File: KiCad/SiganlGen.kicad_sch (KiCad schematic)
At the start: 1 part, among them J1 Barrel_Jack_MountingPin

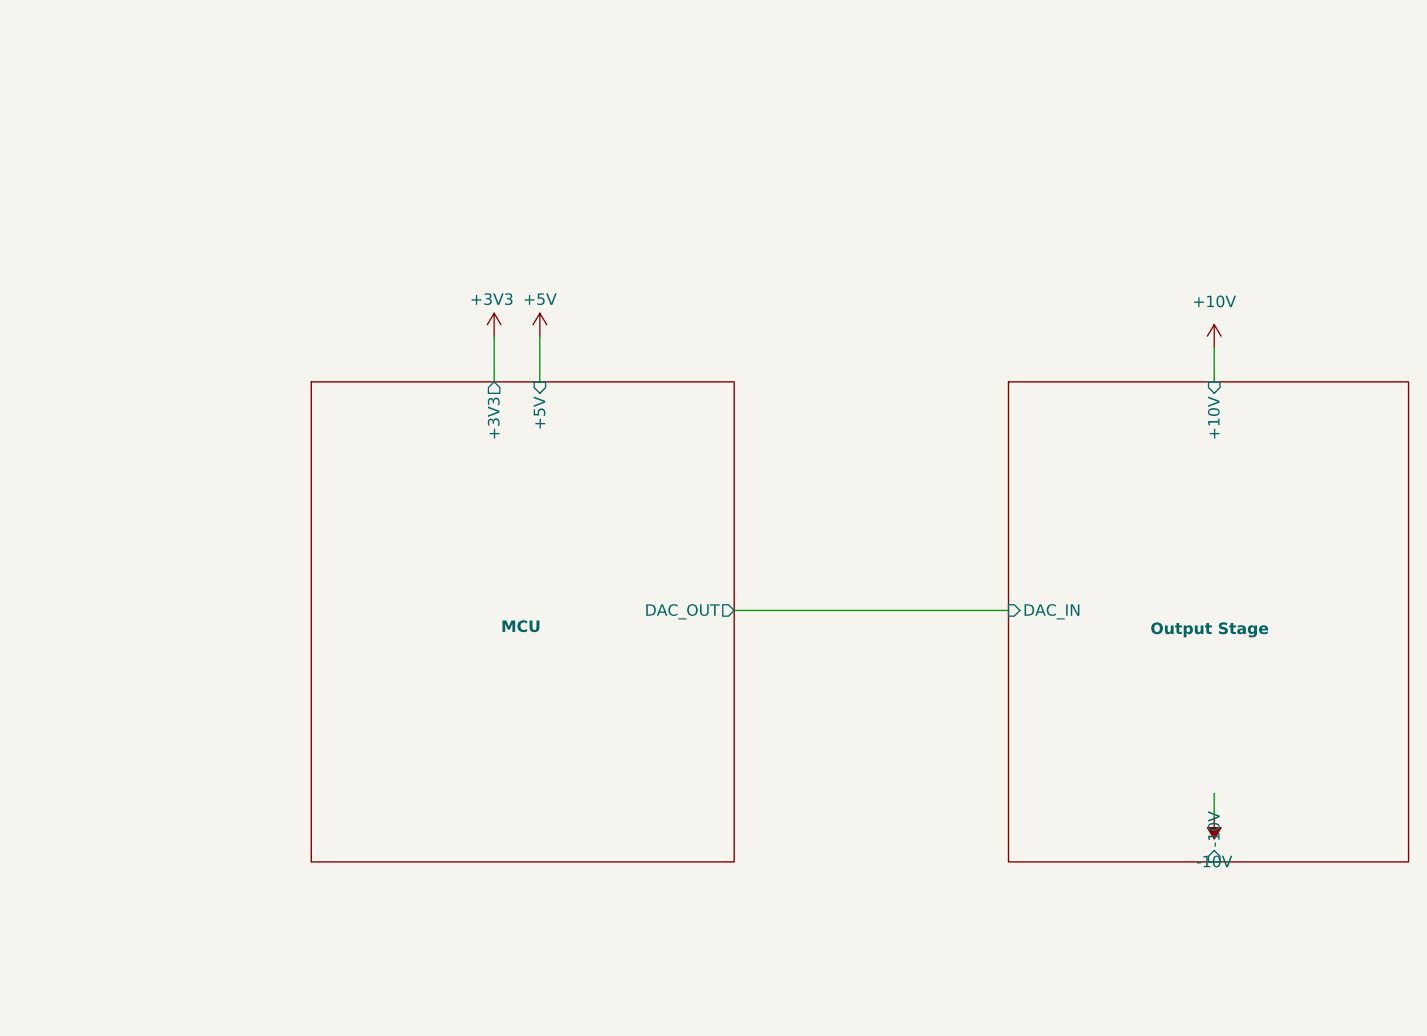
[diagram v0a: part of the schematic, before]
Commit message: minor changes
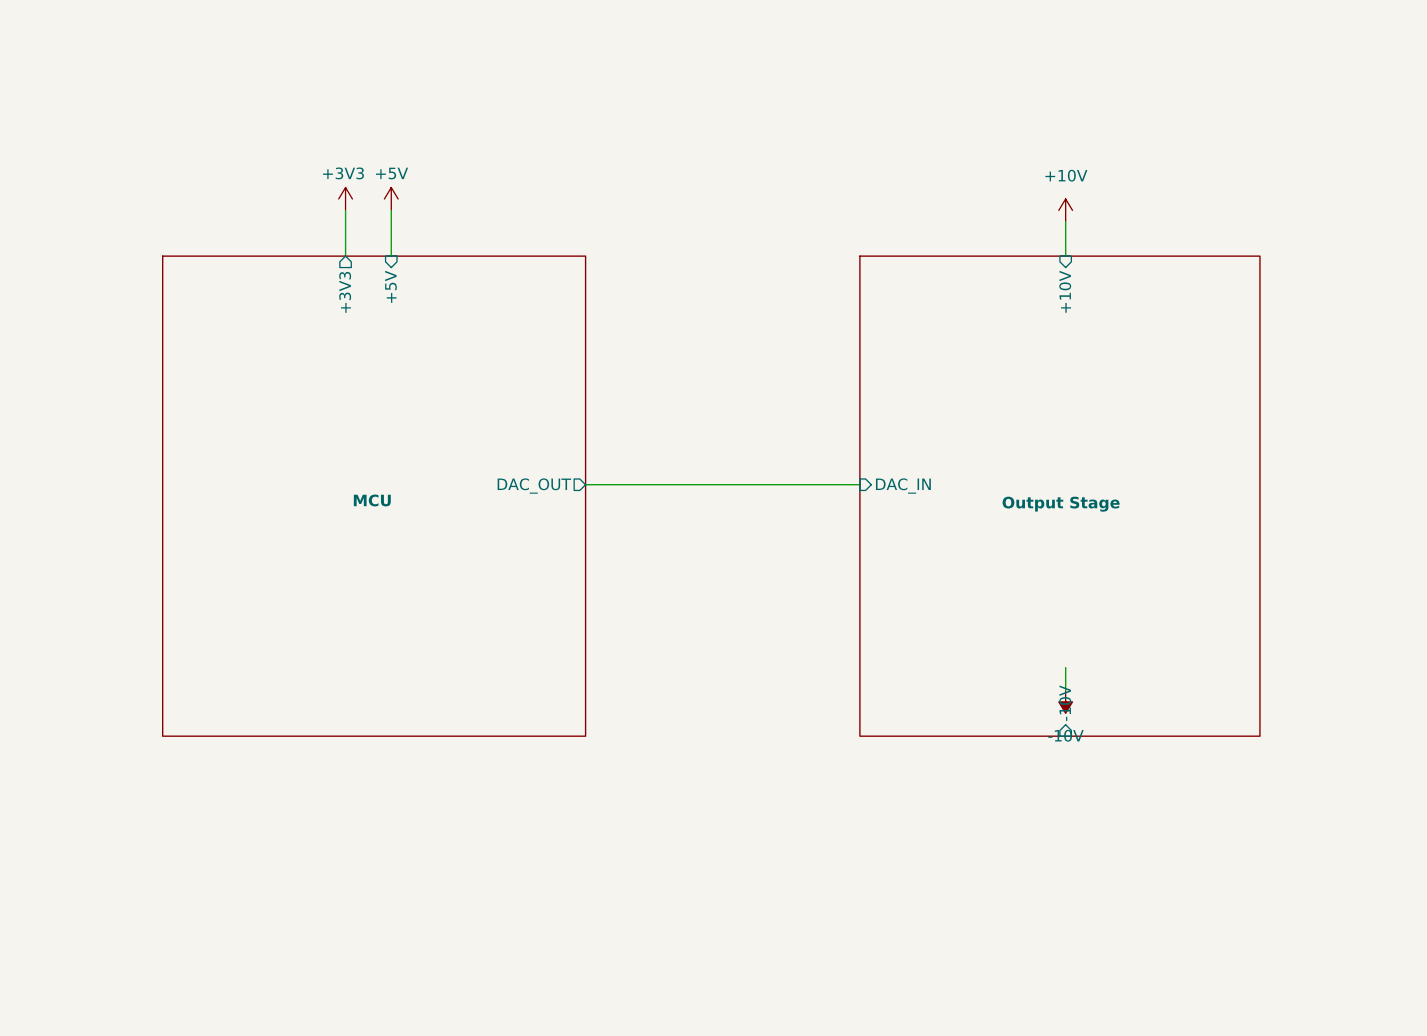
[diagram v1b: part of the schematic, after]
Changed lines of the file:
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@@
 	(wire
 		(pts
-			(xy 195.58 99.06) (xy 226.06 99.06)
+			(xy 179.07 85.09) (xy 209.55 85.09)
 		)
 		(stroke
@@
 	(wire
 		(pts
-			(xy 173.99 68.58) (xy 173.99 73.66)
+			(xy 157.48 54.61) (xy 157.48 59.69)
 		)
 		(stroke
@@
 	(wire
 		(pts
-			(xy 248.92 119.38) (xy 248.92 121.92)
-		)
-		(stroke
-			(width 0)
-			(type default)
-		)
-	)
-	(wire
-		(pts
-			(xy 168.91 68.58) (xy 168.91 73.66)
+			(xy 232.41 105.41) (xy 232.41 107.95)
+		)
+		(stroke
+			(width 0)
+			(type default)
+		)
+	)
+	(wire
+		(pts
+			(xy 152.4 54.61) (xy 152.4 59.69)
 		)
 		(stroke
@@
 	(wire
 		(pts
-			(xy 248.92 69.85) (xy 248.92 73.66)
+			(xy 232.41 55.88) (xy 232.41 59.69)
 		)
 		(stroke
@@
 	(symbol
 		(lib_id "power:+3V3")
-		(at 168.91 68.58 0)
+		(at 152.4 54.61 0)
 		(unit 1)
 		(exclude_from_sim no)
@@
 		(dnp no)
 		(property "Reference" "#PWR011"
-			(at 168.91 72.39 0)
+			(at 152.4 58.42 0)
 			(effects
 				(font
@@
 		)
 		(property "Value" "+3V3"
-			(at 168.656 64.516 0)
+			(at 152.146 50.546 0)
 			(effects
 				(font
@@
 		)
 		(property "Footprint" ""
-			(at 168.91 68.58 0)
+			(at 152.4 54.61 0)
 			(effects
 				(font
@@
 		)
 		(property "Datasheet" ""
-			(at 168.91 68.58 0)
+			(at 152.4 54.61 0)
 			(effects
 				(font
@@
 		)
 		(property "Description" "Power symbol creates a global label with name \"+3V3\""
-			(at 168.91 68.58 0)
+			(at 152.4 54.61 0)
 			(effects
 				(font
@@
 	(symbol
 		(lib_id "power:+5V")
-		(at 173.99 68.58 0)
+		(at 157.48 54.61 0)
 		(unit 1)
 		(exclude_from_sim no)
@@
 		(dnp no)
 		(property "Reference" "#PWR016"
-			(at 173.99 72.39 0)
+			(at 157.48 58.42 0)
 			(effects
 				(font
@@
 		)
 		(property "Value" "+5V"
-			(at 173.99 64.516 0)
+			(at 157.48 50.546 0)
 			(effects
 				(font
@@
 		)
 		(property "Footprint" ""
-			(at 173.99 68.58 0)
+			(at 157.48 54.61 0)
 			(effects
 				(font
@@
 		)
 		(property "Datasheet" ""
-			(at 173.99 68.58 0)
+			(at 157.48 54.61 0)
 			(effects
 				(font
@@
 		)
 		(property "Description" "Power symbol creates a global label with name \"+5V\""
-			(at 173.99 68.58 0)
+			(at 157.48 54.61 0)
 			(effects
 				(font
@@
 	(symbol
 		(lib_id "power:+10V")
-		(at 248.92 69.85 0)
+		(at 232.41 55.88 0)
 		(unit 1)
 		(exclude_from_sim no)
@@
 		(fields_autoplaced yes)
 		(property "Reference" "#PWR021"
-			(at 248.92 73.66 0)
+			(at 232.41 59.69 0)
 			(effects
 				(font
@@
 		)
 		(property "Value" "+10V"
-			(at 248.92 64.77 0)
+			(at 232.41 50.8 0)
 			(effects
 				(font
@@
 		)
 		(property "Footprint" ""
-			(at 248.92 69.85 0)
+			(at 232.41 55.88 0)
 			(effects
 				(font
@@
 		)
 		(property "Datasheet" ""
-			(at 248.92 69.85 0)
+			(at 232.41 55.88 0)
 			(effects
 				(font
@@
 		)
 		(property "Description" "Power symbol creates a global label with name \"+10V\""
-			(at 248.92 69.85 0)
+			(at 232.41 55.88 0)
 			(effects
 				(font
@@
 	(symbol
 		(lib_id "power:-10V")
-		(at 248.92 121.92 180)
+		(at 232.41 107.95 180)
 		(unit 1)
 		(exclude_from_sim no)
@@
 		(fields_autoplaced yes)
 		(property "Reference" "#PWR018"
-			(at 248.92 118.11 0)
+			(at 232.41 104.14 0)
 			(effects
 				(font
@@
 		)
 		(property "Value" "-10V"
-			(at 248.92 127 0)
+			(at 232.41 113.03 0)
 			(effects
 				(font
@@
 		)
 		(property "Footprint" ""
-			(at 248.92 121.92 0)
+			(at 232.41 107.95 0)
 			(effects
 				(font
@@
 		)
 		(property "Datasheet" ""
-			(at 248.92 121.92 0)
+			(at 232.41 107.95 0)
 			(effects
 				(font
@@
 		)
 		(property "Description" "Power symbol creates a global label with name \"-10V\""
-			(at 248.92 121.92 0)
+			(at 232.41 107.95 0)
 			(effects
 				(font
@@
 	)
 	(sheet
-		(at 148.59 73.66)
+		(at 132.08 59.69)
 		(size 46.99 53.34)
 		(stroke
@@
 		)
 		(property "Sheetname" "MCU"
-			(at 169.672 101.6 0)
+			(at 153.162 87.63 0)
 			(effects
 				(font
@@
 		)
 		(property "Sheetfile" "MCU.kicad_sch"
-			(at 148.59 127.5846 0)
+			(at 132.08 113.6146 0)
 			(effects
 				(font
@@
 		)
 		(pin "+3V3" output
-			(at 168.91 73.66 90)
+			(at 152.4 59.69 90)
 			(effects
 				(font
@@
 		)
 		(pin "+5V" input
-			(at 173.99 73.66 90)
+			(at 157.48 59.69 90)
 			(effects
 				(font
@@
 		)
 		(pin "DAC_OUT" output
-			(at 195.58 99.06 0)
+			(at 179.07 85.09 0)
 			(effects
 				(font
@@
 	)
 	(sheet
-		(at 226.06 73.66)
+		(at 209.55 59.69)
 		(size 44.45 53.34)
 		(stroke
@@
 		)
 		(property "Sheetname" "Output Stage"
-			(at 248.412 101.092 0)
+			(at 231.902 87.122 0)
 			(effects
 				(font
@@
 		)
 		(property "Sheetfile" "OutputStage.kicad_sch"
-			(at 226.06 119.9646 0)
+			(at 209.55 105.9946 0)
 			(effects
 				(font
@@
 		)
 		(pin "DAC_IN" input
-			(at 226.06 99.06 180)
+			(at 209.55 85.09 180)
 			(effects
 				(font
@@
 		)
 		(pin "-10V" input
-			(at 248.92 127 270)
+			(at 232.41 113.03 270)
 			(effects
 				(font
@@
 		)
 		(pin "+10V" input
-			(at 248.92 73.66 90)
-			(effects
-				(font
+			(at 232.41 59.69 90)
+			(effects
+				(font
